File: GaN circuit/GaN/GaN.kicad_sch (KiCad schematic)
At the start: 9 parts, among them IC1 LTC7891RUFDM#PBF

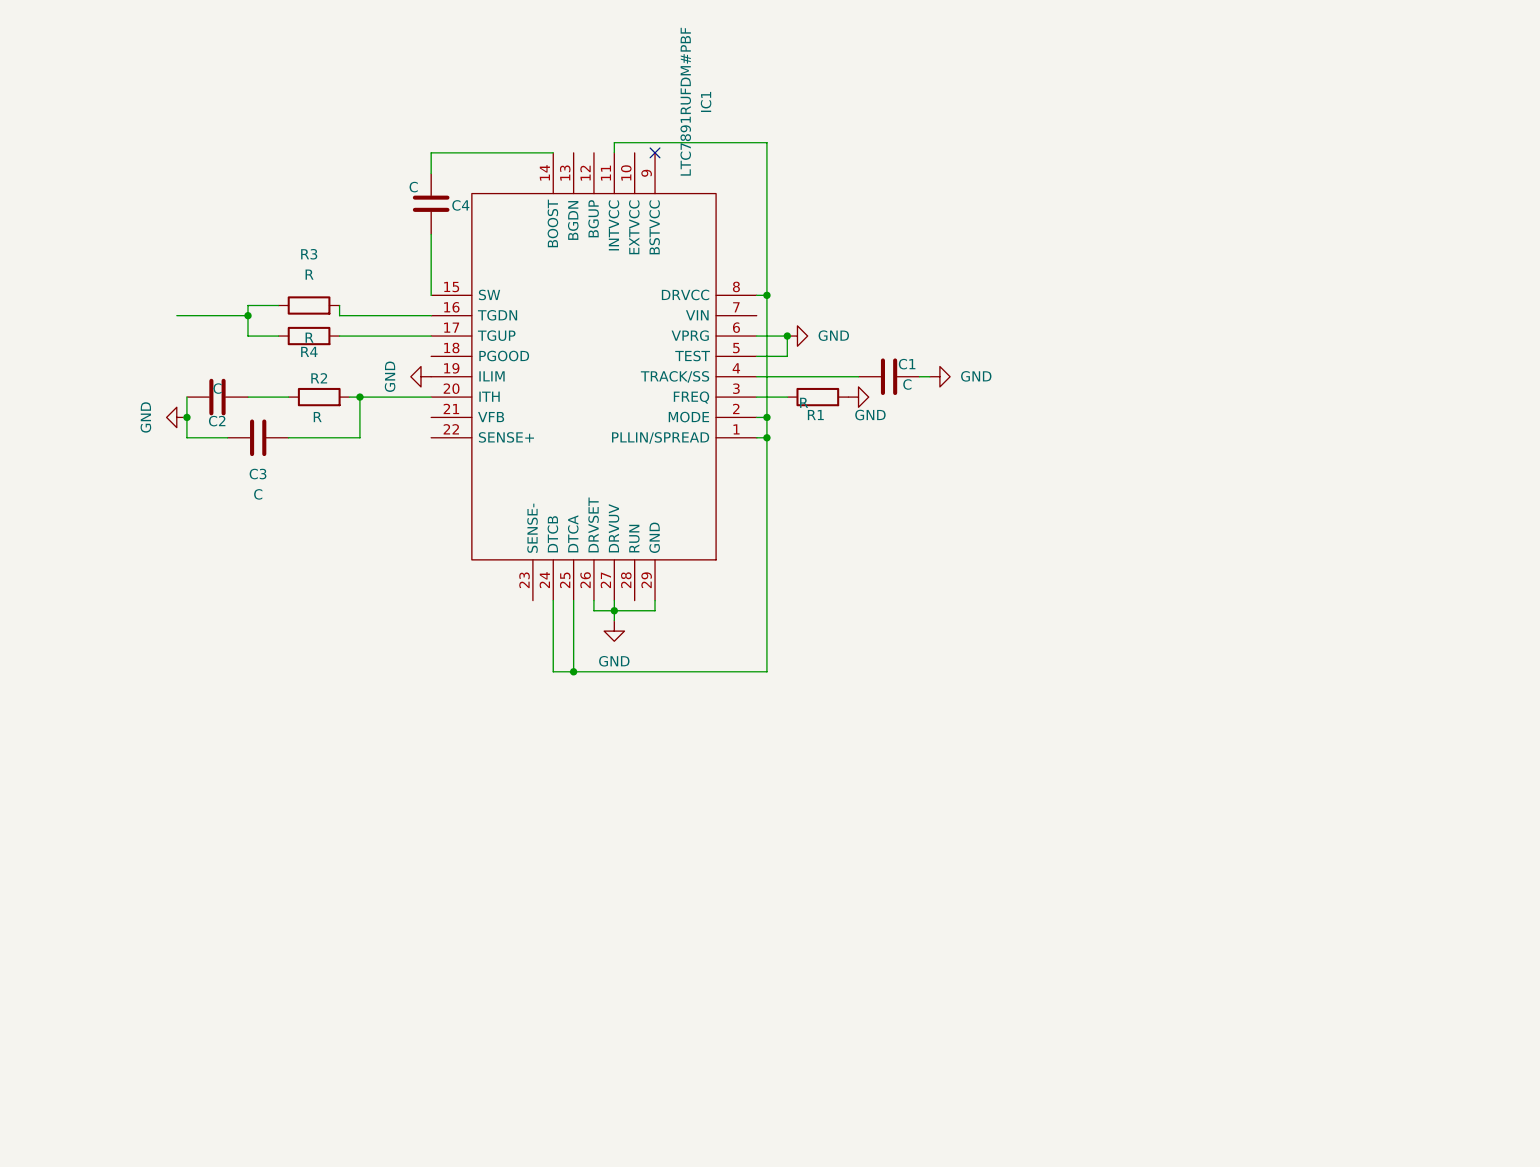
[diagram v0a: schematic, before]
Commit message: Finished GaN schematic
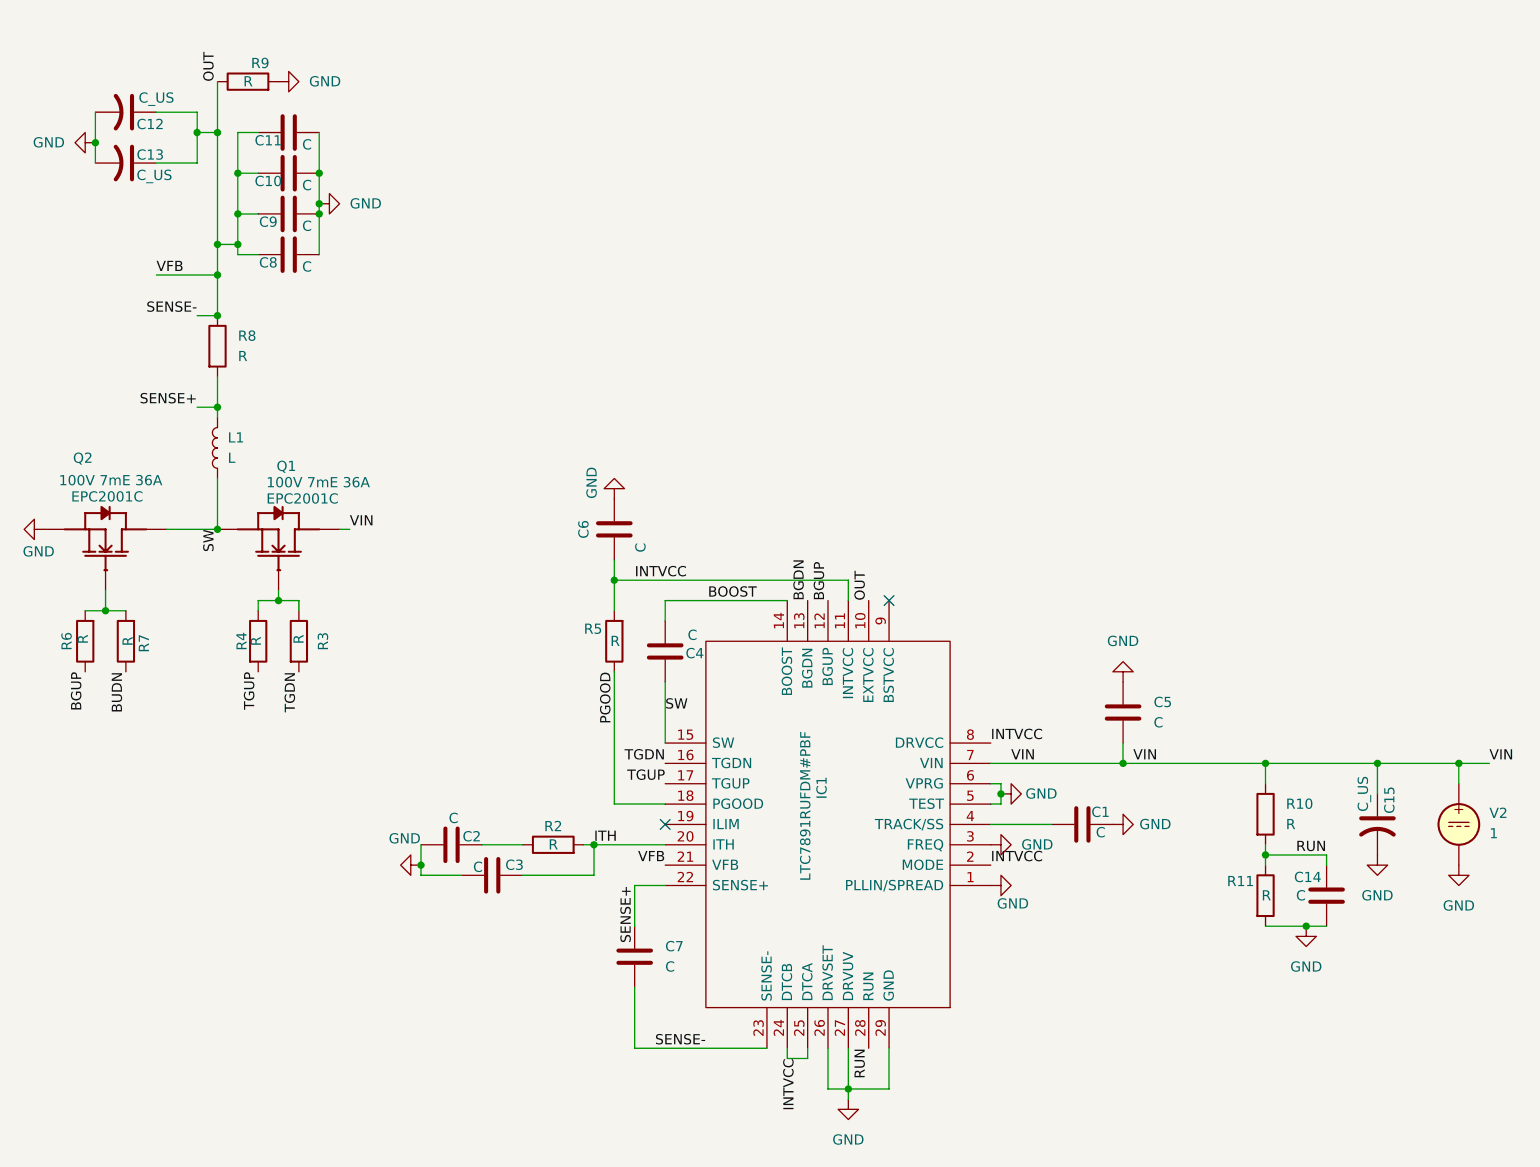
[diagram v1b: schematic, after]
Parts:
- removed R1: R, symbol Device:R
- added C10, C11, C14, C5, C6, C7, C8, C9: C, symbol Device:C
- added C12, C13, C15: C_US, symbol Device:C_US
- added L1: L, symbol Device:L
- added Q1, Q2: EPC2001C, EPC_FETs:D0188, symbol EPC_FETs:EPC2001C
- added R10, R11, R5, R6, R7, R8, R9: R, symbol Device:R
- added V2: 1, symbol Simulation_SPICE:VDC
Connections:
- net GND: now also IC1.1 (PLLIN/SPREAD), IC1.3 (FREQ), C10.2, C11.2, C12.2, C13.2, C14.2, C15.2, C5.1, C6.1, C8.2, C9.2, Q2.10 (S4), Q2.2 (Sub), Q2.4 (S1), Q2.6 (S2), Q2.8 (S3), R11.2, R9.2, V2.2; no longer IC1.19 (ILIM)
- net ITH: now reaches C3.2, IC1.20 (ITH), R2.2
- net at R3.1, R4.1: now also Q1.1 (G)
- net TGUP: now reaches IC1.17 (TGUP), R4.2
- net INTVCC: now reaches IC1.11 (INTVCC), IC1.2 (MODE), IC1.24 (DTCB), IC1.25 (DTCA), IC1.8 (DRVCC)
- net INTVCC: now also C6.2, R5.2; no longer IC1.1 (PLLIN/SPREAD)
- net OUT: now reaches IC1.10 (EXTVCC)
- net OUT: now also IC1.21 (VFB), IC1.23 (SENSE-), C10.1, C11.1, C12.1, C13.1, C7.2, C8.1, C9.1, R8.1, R9.1
- net BGUP: now reaches IC1.12 (BGUP)
- net BGUP: now also R6.1
- net BGDN: now reaches IC1.13 (BGDN)
- net BOOST: now reaches C4.1, IC1.14 (BOOST)
- net SW: now reaches C4.2, IC1.15 (SW)
- net SW: now also L1.1, Q1.10 (S4), Q1.2 (Sub), Q1.4 (S1), Q1.6 (S2), Q1.8 (S3), Q2.11 (D5), Q2.3 (D1), Q2.5 (D2), Q2.7 (D3), Q2.9 (D4)
- net TGDN: now reaches IC1.16 (TGDN), R3.2
- net PGOOD: now reaches IC1.18 (PGOOD)
- net PGOOD: now also R5.1
- net SENSE+: now reaches IC1.22 (SENSE+)
- net SENSE+: now also C7.1, L1.2, R8.2
- net RUN: now reaches IC1.28 (RUN)
- net RUN: now also C14.1, R10.2, R11.1
- net VIN: now reaches IC1.7 (VIN)
- net VIN: now also C15.1, C5.2, Q1.11 (D5), Q1.3 (D1), Q1.5 (D2), Q1.7 (D3), Q1.9 (D4), R10.1, V2.1
- new net: Q2.1 (G), R6.2, R7.2
- new net BUDN: R7.1
- no-connect marks 1 -> 2
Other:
- moved on the sheet: C1, C2, C3, C4, IC1, R2, R3, R4
